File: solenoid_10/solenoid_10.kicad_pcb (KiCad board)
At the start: 4 copper layers, 233 x 48.5 mm, 129 parts, among them J1 Conn_01x12_Pin, J10 1217080-1, J11 1217080-1, J12 1217080-1, J13 1217080-1, J14 1217080-1, J15 1217080-1, J16 1217080-1, J17 1217080-1, J18 1217080-1, J19 1217080-1, J2 1217080-1, J20 1217080-1, J21 1217080-1, J3 1217080-1, J4 1217080-1, J5 1217080-1, J6 1217080-1, J7 1217080-1, J8 1217080-1, J9 1217080-1, Q1 AO4486, Q10 AO4486, Q11 AO4486, Q2 BT148W-600R, Q3 AO4486, Q4 AO4486, Q5 AO4486, Q6 AO4486, Q7 AO4486, Q8 AO4486, Q9 AO4486, U1 XL1509-5.0

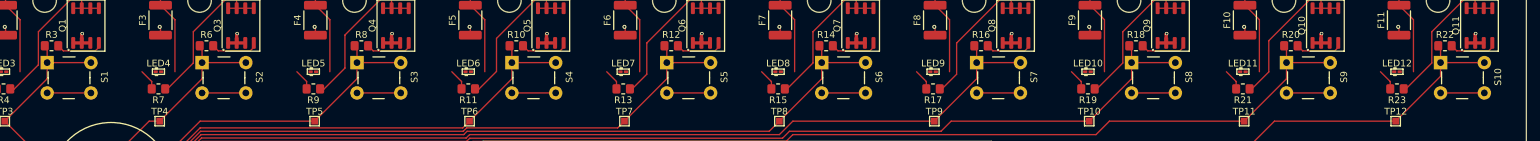
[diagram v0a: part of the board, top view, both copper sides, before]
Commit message: Appended change.
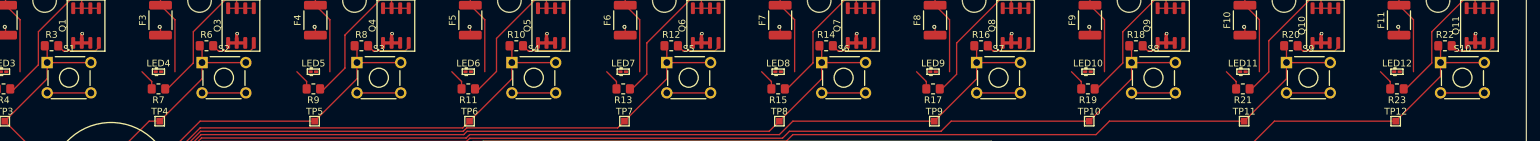
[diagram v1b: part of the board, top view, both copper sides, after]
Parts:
- S1, S10, S2, S3, S4, S5, S6, S7, S8, S9: footprint digikey-footprints:Switch_Tactile_THT_B3F-1xxx -> solenoid_fp:SW_TH_Tactile_Omron_B3F-10xx
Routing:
- net /VGATE: track 81.4 -> 16.4 mm
- net /CH6_IN: track 121.6 -> 128.1 mm
- net /CH9_IN: track 197.9 -> 204.4 mm
- net /CH8_IN: track 172.0 -> 178.5 mm
- net /CH7_IN: track 146.5 -> 153.0 mm
- net /CH5_IN: track 99.4 -> 105.9 mm
- net /CH4_IN: track 74.4 -> 80.9 mm
- net /CH3_IN: track 52.2 -> 58.7 mm
- net /CH1_IN: track 37.0 -> 43.5 mm
- net /CH10_IN: track 223.7 -> 230.2 mm
- net /CH2_IN: track 31.1 -> 37.6 mm
